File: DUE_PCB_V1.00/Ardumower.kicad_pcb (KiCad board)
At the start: 2 copper layers, 169.8 x 97 mm, 86 parts, among them J1 9V IN, J10 Sonar_R, J11 Sonar_C, J12 Sonar_L, J13 P_Right, J14 Buzzer, J15 Button, J16 US1, J17 US2, J18 US3, J19 P_Left, J2 I2C0_1, J20 Remote, J21 PCB_2, J22 Ser0, J23 Ser1, J24 Ser2, J25 5V IN, J26 Cutter1, J27 MotorR, J28 MotorL, J29 3.3V IN, J3 I2C0_2, J30 I2C1_2, J31 Ser3, J32 24V In, J33 ReserveD8, J34 ReserveD9, J35 ReserveD49, J36 ReserveA10, J37 RPM_Mow, J38 ODO_Left, J39 ODO_Right, J4 I2C1_1, J40 Motor_Right, J41 Motor_Left, J42 Cutter, J5 Bumper, J6 Drop_Left, J7 Drop_Right, J8 Tilt, J9 Rain, U1 MC33926, U2 MC33926

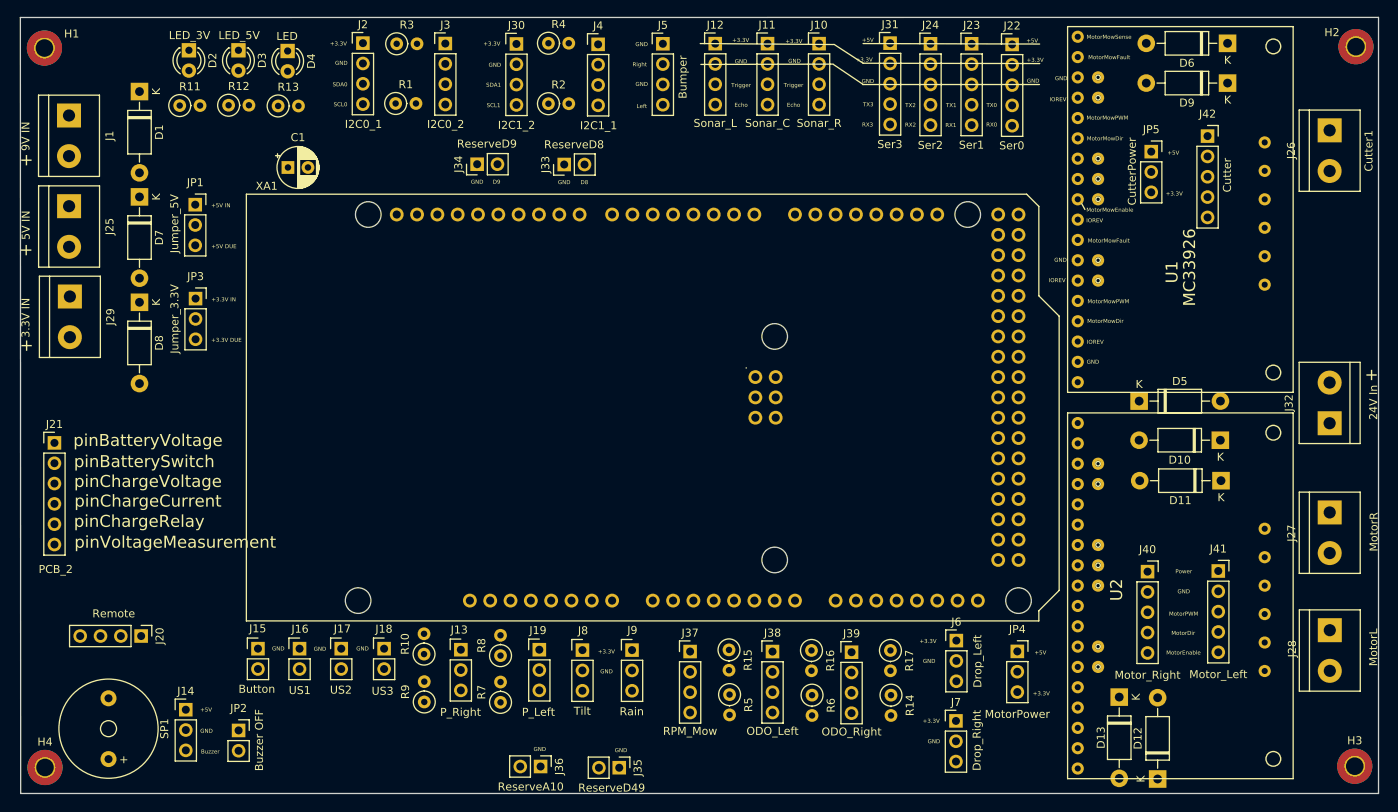
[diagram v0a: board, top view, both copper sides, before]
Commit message: First Route Test
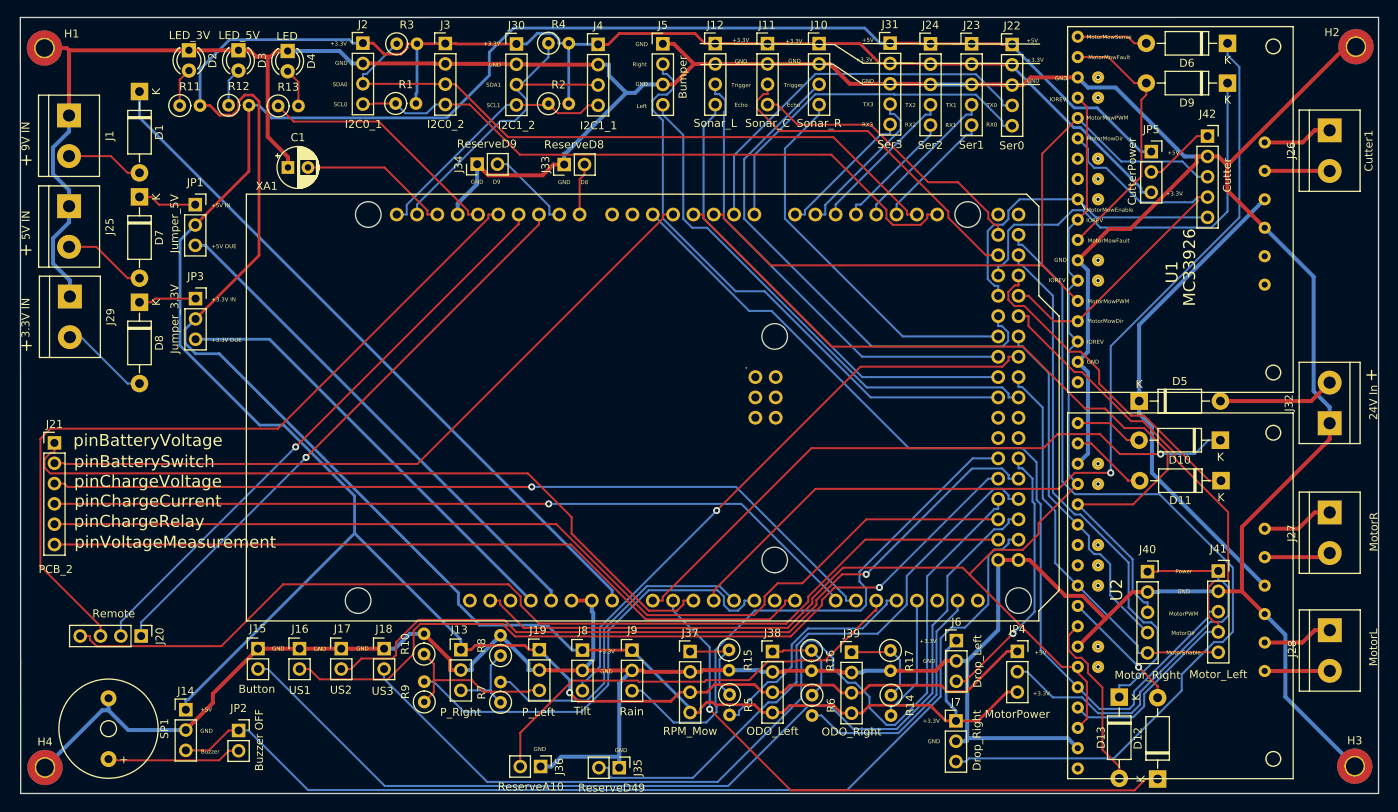
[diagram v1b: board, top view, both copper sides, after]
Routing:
- net GND: track 0.00 -> 656.8 mm
- net +3V3: track 0.00 -> 336.2 mm
- net +5V: track 0.00 -> 323.6 mm, vias 0 -> 1
- net IOREV: track 0.00 -> 163.4 mm
- net pinBuzzer: track 0.00 -> 129.3 mm
- net pinChargeRelay: track 0.00 -> 128.2 mm
- net pinRemoteSwitch: track 0.00 -> 126.1 mm
- net pinButton: track 0.00 -> 125.1 mm
- net pinUserSwitch3: track 0.00 -> 121.3 mm
- net pinMotorMowSense: track 0.00 -> 117.9 mm, vias 0 -> 1
- net pinMotorLeftPWM: track 0.00 -> 116.1 mm
- net pinDropRight: track 0.00 -> 109.7 mm
- net pinChargeVoltage: track 0.00 -> 106.5 mm, vias 0 -> 1
- net pinMotorRightPWM: track 0.00 -> 104.5 mm
- net pinChargeCurrent: track 0.00 -> 102.8 mm, vias 0 -> 1
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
